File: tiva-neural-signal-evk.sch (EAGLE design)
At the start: 93 parts, among them IC1 TM4C123G, IC2 TLV70233, IC3 INA2332, IC4 OPA2320, IC5 OPA2320, IC6 INA2332, IC7 OPA2320, IC8 OPA2320, X1 USB, X2 MICROSD, Y1 16MHz, Y2 32.768kHz

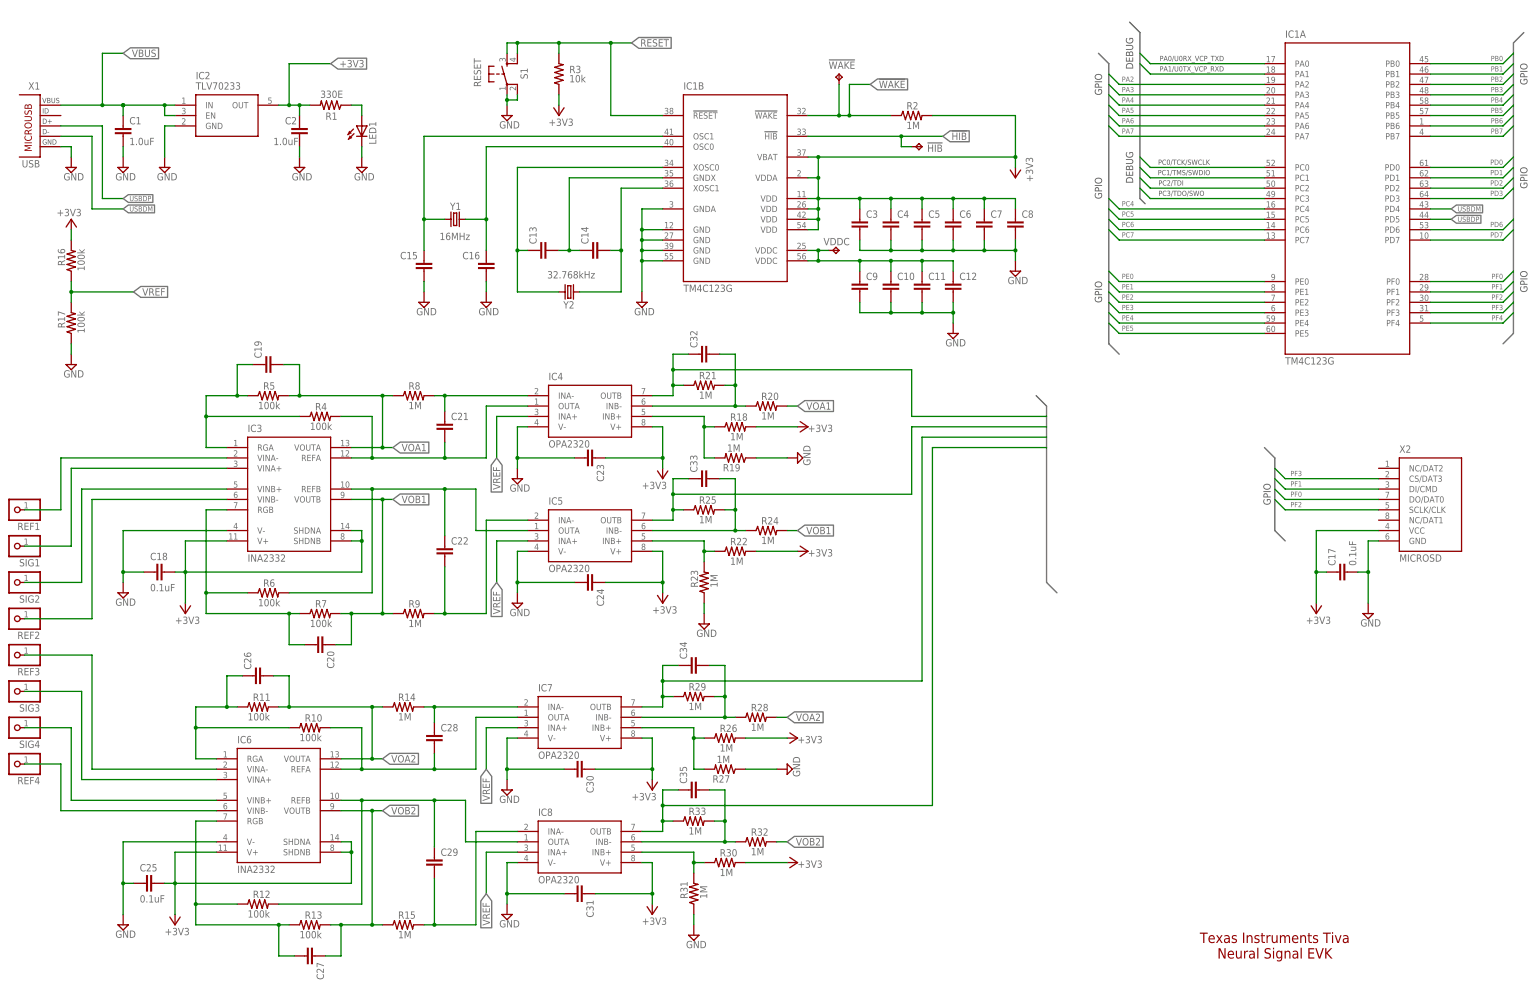
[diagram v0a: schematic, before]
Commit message: Revert "Revert "added everything. initial routing complete with signal planes""
This reverts commit d55bffc2993c446258426b3721d1dfd936908fa6.
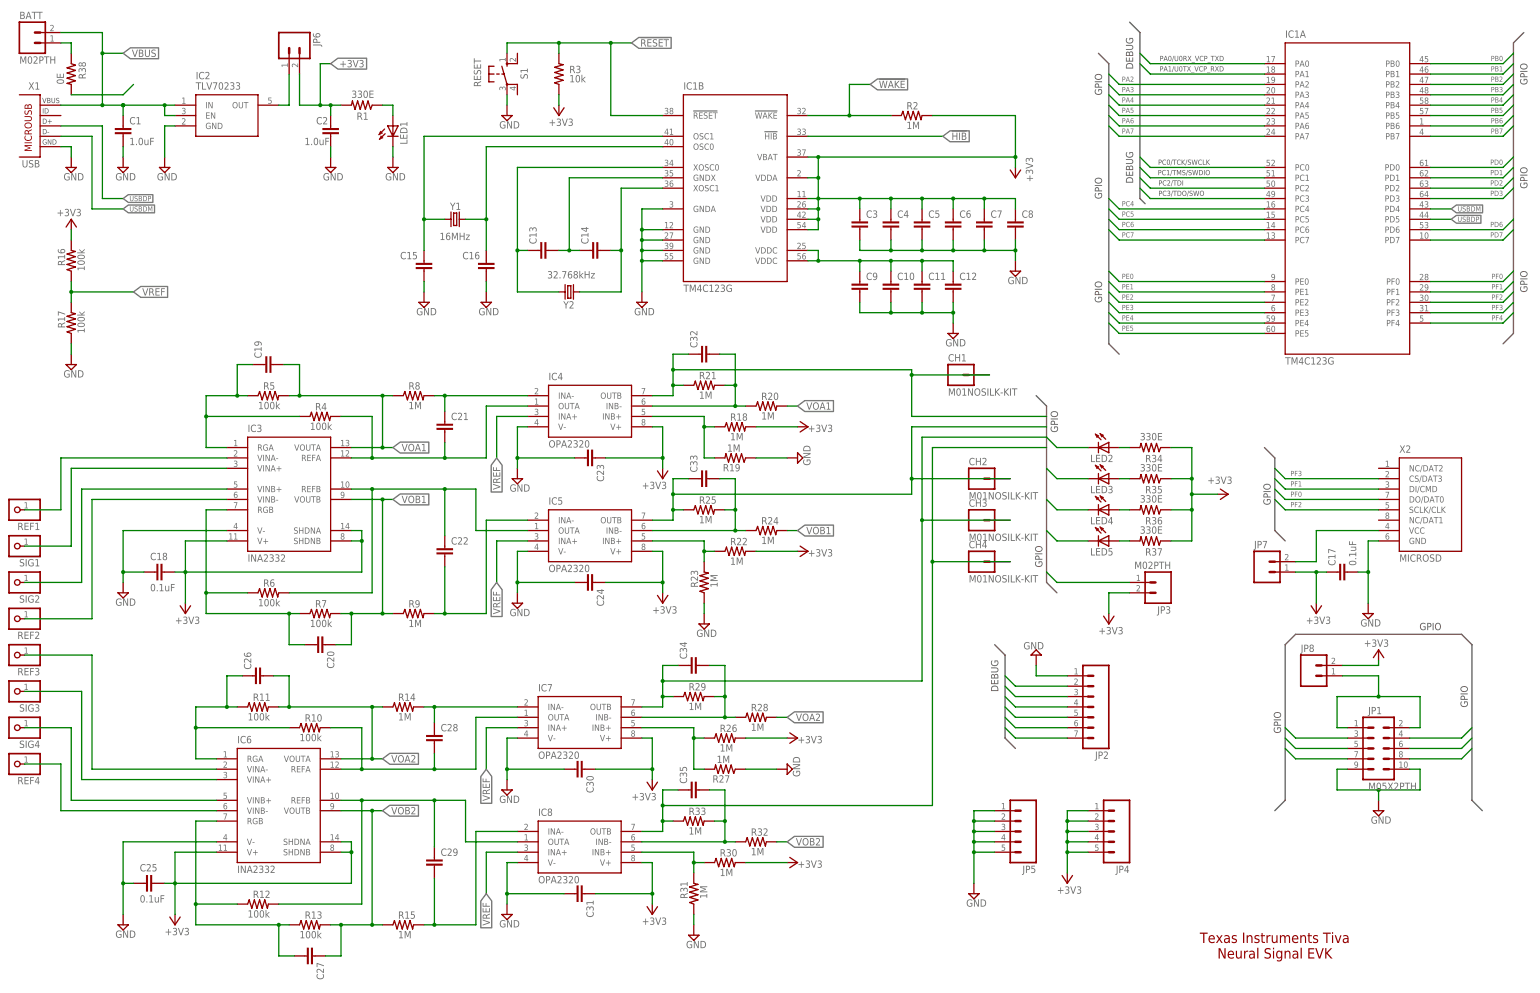
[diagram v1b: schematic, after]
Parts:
- removed !HIB!, !WAKE!, VDDC: TPB1,27, testpad:TPB1,27
- added BATT, JP3: M02PTH, SparkFun-Connectors:M02PTH
- added CH1, CH2, CH3, CH4: M01NOSILK-KIT, SparkFun-Connectors:M01NOSILK-KIT
- added JP1: M05X2PTH, SparkFun-Connectors:M05X2PTH
- added JP2: (no value), SparkFun-Connectors:M07
- added JP4, JP5: (no value), SparkFun-Connectors:M05PTH
- added JP6, JP7, JP8: M021X02_NO_SILK, SparkFun-Connectors:M021X02_NO_SILK
- added LED2, LED3, LED4, LED5: (no value), led:LEDCHIP-LED0603
- added R34, R35, R36, R37: 330E, rcl:R-US_R0603
- added R38: 0E, rcl:R-US_R0603
- S1: device mor307:6MM_SWITCH6MM_SWITCH -> CEDTv82:10-XX
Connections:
- new net AGND: C18.2, C23.2, C24.2, C25.2, C30.2, C31.2, IC3.V-, IC4.V-, IC5.V-, IC6.V-, IC7.V-, IC8.V-, JP5.1, JP5.2, JP5.3, JP5.4, JP5.5, R17.1, R19.1, R23.1, R27.1, R31.1, R38.2
- new net N$31: LED2.A, R34.2
- new net N$35: LED3.A, R35.2
- new net N$36: LED4.A, R36.2
- new net N$37: LED5.A, R37.2
- new net N$38: IC2.OUT, JP6.1
- new net N$39: BATT.1, R38.1
- new net N$40: JP7.2, X2.VCC
- new net N$41: JP1.1, JP1.2, JP8.1
- net !HIB!: no longer !HIB!.TP
- net !RESET!: no longer S1.S1
- net !WAKE!: no longer !WAKE!.TP
- net +3V3: now also JP3.2, JP4.1, JP4.2, JP4.3, JP4.4, JP4.5, JP6.2, JP7.1, JP8.2, R34.1, R35.1, R36.1, R37.1; no longer IC2.OUT, X2.VCC
- net GND: now also JP1.10, JP1.9, JP2.1; no longer C18.2, C23.2, C24.2, C25.2, C30.2, C31.2, IC3.V-, IC4.V-, IC5.V-, IC6.V-, IC7.V-, IC8.V-, R17.1, R19.1, R23.1, R27.1, R31.1, S1.P1
- net PA0: now also JP2.2
- net PA1: now also JP2.3
- net PB0: now also LED2.C
- net PB1: now also LED3.C
- net PB2: now also LED4.C
- net PB3: now also LED5.C
- net PB6: now also JP1.3
- net PB7: now also JP1.8
- net PC0: now also JP2.4
- net PC1: now also JP2.5
- net PC2: now also JP2.6
- net PC3: now also JP2.7
- net PD0: now also JP1.5
- net PD1: now also JP1.4
- net PD2: now also JP1.7
- net PD3: now also JP1.6
- net PE0: now also CH4.1
- net PE1: now also CH3.1
- net PE2: now also CH2.1
- net PE3: now also CH1.1
- net PF3: now also JP3.1
- net VBUS: now also BATT.2
- net VDDC: no longer VDDC.TP
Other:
- moved on the sheet: C2, LED1, R1

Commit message: Revert "added everything. initial routing complete with signal planes"
This reverts commit afc261f9183dc80193b5e18bad7752eddb98d99b.
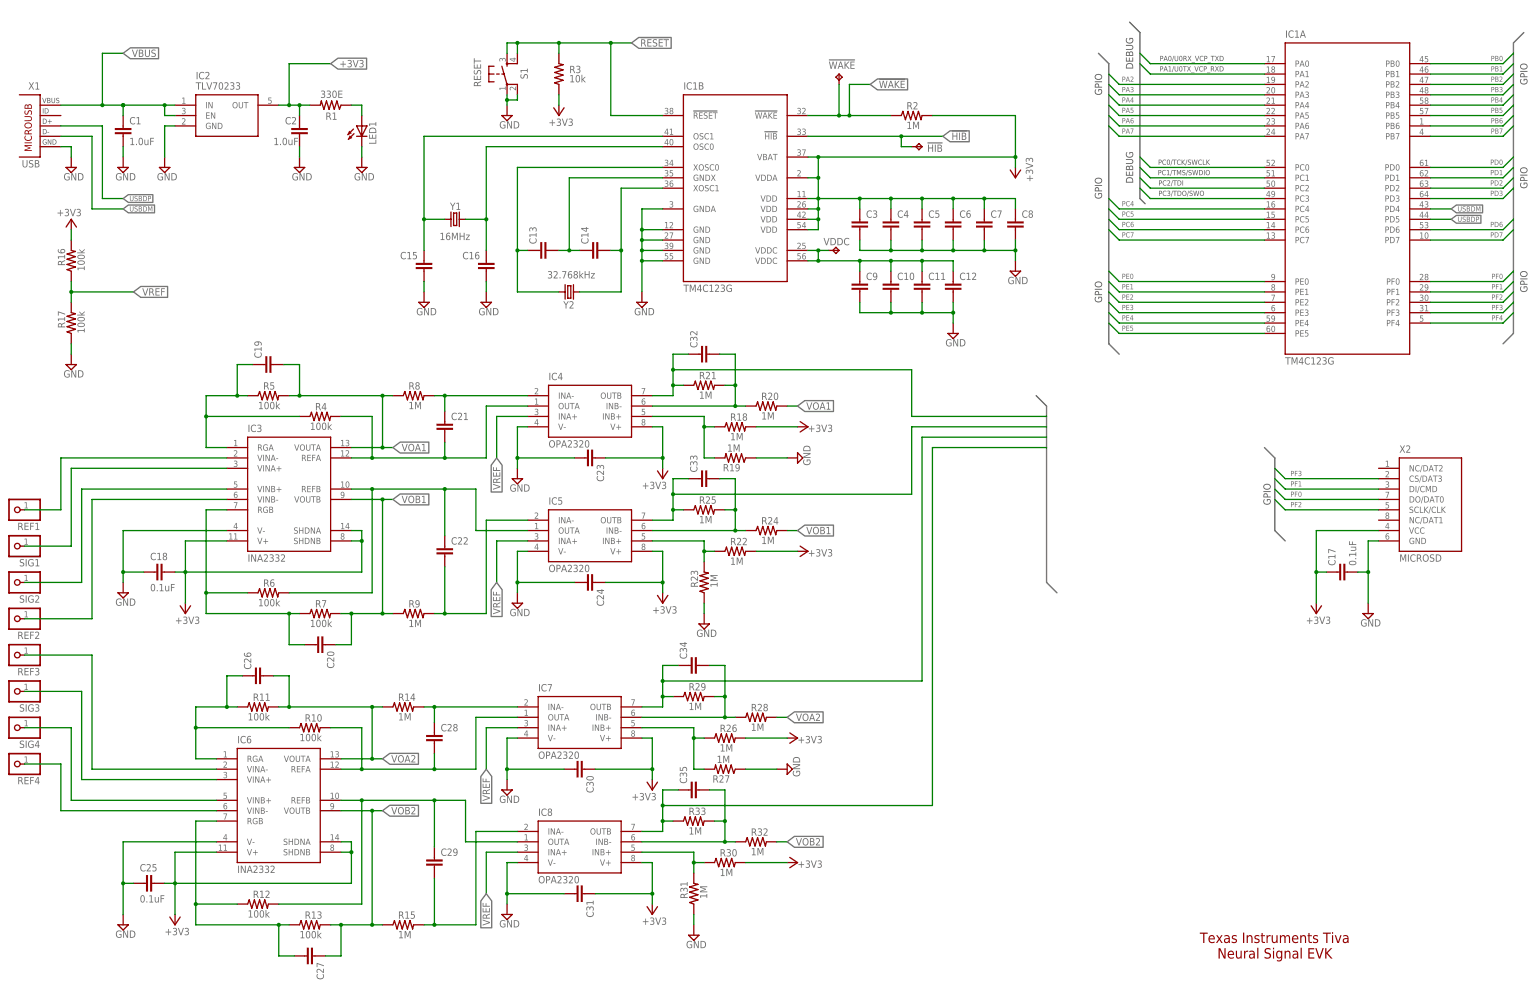
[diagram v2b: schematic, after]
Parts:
- removed BATT, JP3: M02PTH, SparkFun-Connectors:M02PTH
- removed CH1, CH2, CH3, CH4: M01NOSILK-KIT, SparkFun-Connectors:M01NOSILK-KIT
- removed JP1: M05X2PTH, SparkFun-Connectors:M05X2PTH
- removed JP2: (no value), SparkFun-Connectors:M07
- removed JP4, JP5: (no value), SparkFun-Connectors:M05PTH
- removed JP6, JP7, JP8: M021X02_NO_SILK, SparkFun-Connectors:M021X02_NO_SILK
- removed LED2, LED3, LED4, LED5: (no value), led:LEDCHIP-LED0603
- removed R34, R35, R36, R37: 330E, rcl:R-US_R0603
- removed R38: 0E, rcl:R-US_R0603
- added !HIB!, !WAKE!, VDDC: TPB1,27, testpad:TPB1,27
- S1: device CEDTv82:10-XX -> mor307:6MM_SWITCH6MM_SWITCH
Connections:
- removed net AGND: C18.2, C23.2, C24.2, C25.2, C30.2, C31.2, IC3.V-, IC4.V-, IC5.V-, IC6.V-, IC7.V-, IC8.V-, JP5.1, JP5.2, JP5.3, JP5.4, JP5.5, R17.1, R19.1, R23.1, R27.1, R31.1, R38.2
- removed net N$31: LED2.A, R34.2
- removed net N$35: LED3.A, R35.2
- removed net N$36: LED4.A, R36.2
- removed net N$37: LED5.A, R37.2
- removed net N$38: IC2.OUT, JP6.1
- removed net N$39: BATT.1, R38.1
- removed net N$40: JP7.2, X2.VCC
- removed net N$41: JP1.1, JP1.2, JP8.1
- net !HIB!: now also !HIB!.TP
- net !RESET!: now also S1.S1
- net !WAKE!: now also !WAKE!.TP
- net +3V3: now also IC2.OUT, X2.VCC; no longer JP3.2, JP4.1, JP4.2, JP4.3, JP4.4, JP4.5, JP6.2, JP7.1, JP8.2, R34.1, R35.1, R36.1, R37.1
- net GND: now also C18.2, C23.2, C24.2, C25.2, C30.2, C31.2, IC3.V-, IC4.V-, IC5.V-, IC6.V-, IC7.V-, IC8.V-, R17.1, R19.1, R23.1, R27.1, R31.1, S1.P1; no longer JP1.10, JP1.9, JP2.1
- net PA0: no longer JP2.2
- net PA1: no longer JP2.3
- net PB0: no longer LED2.C
- net PB1: no longer LED3.C
- net PB2: no longer LED4.C
- net PB3: no longer LED5.C
- net PB6: no longer JP1.3
- net PB7: no longer JP1.8
- net PC0: no longer JP2.4
- net PC1: no longer JP2.5
- net PC2: no longer JP2.6
- net PC3: no longer JP2.7
- net PD0: no longer JP1.5
- net PD1: no longer JP1.4
- net PD2: no longer JP1.7
- net PD3: no longer JP1.6
- net PE0: no longer CH4.1
- net PE1: no longer CH3.1
- net PE2: no longer CH2.1
- net PE3: no longer CH1.1
- net PF3: no longer JP3.1
- net VBUS: no longer BATT.2
- net VDDC: now also VDDC.TP
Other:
- moved on the sheet: C2, LED1, R1
